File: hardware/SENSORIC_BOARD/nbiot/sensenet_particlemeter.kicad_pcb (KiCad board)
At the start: 2 copper layers, 63.6 x 72.3 mm, 80 parts, among them J1 CONN_01X01, J11 CONN_01X01, J13 BARREL_JACK, J17 CONN_01X01, J18 CONN_01X01, J19 CONN_01X01, J2 CONN_01X01, J20 CONN_01X01, J21 CONN_01X01, J3 CONN_01X01, J4 CONN_01X01, J5 CONN_01X01, J6 CONN_01X01, J9 CONN_01X01, P1 SMA_mini, P2 SMA_mini, P3 CONN_02X11, P4 USB_B, Q1 Q_NMOS_GSD, SW1 SW_Push, SW2 SW_DIP_x02, U1 MC33063, U10 bme280_barebone, U2 stm32f072, U3 QUECTEL_BC95, U4 SIM, U5 CAT24C02, U7 M10578-A2, U8 LD39050, Y1 8MHz

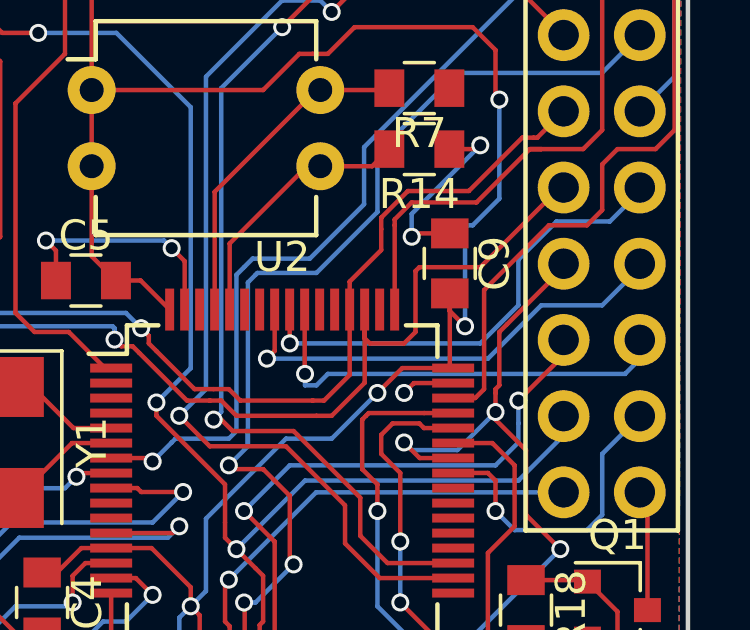
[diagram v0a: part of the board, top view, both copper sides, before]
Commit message: Zaklad nove verze je hotovy, ted jdu udelat vetsi zmeny v napajeni a layoutu, priprava na shield atd.
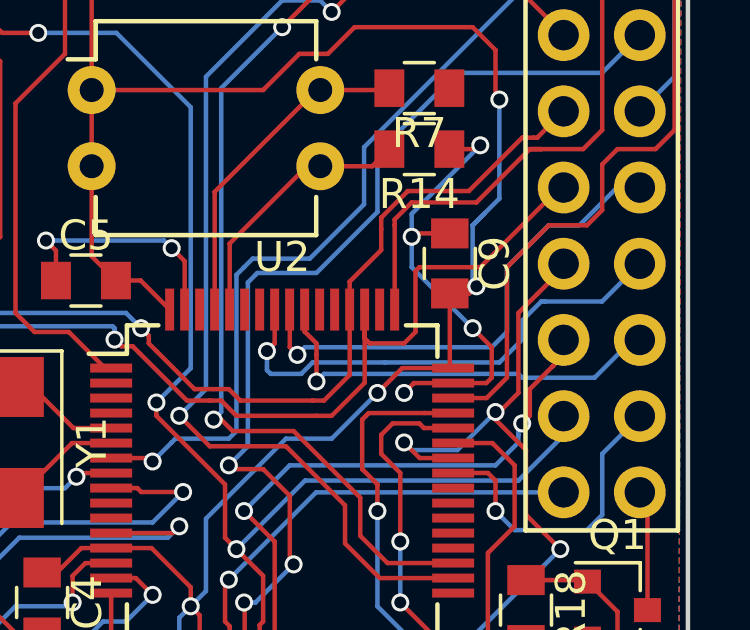
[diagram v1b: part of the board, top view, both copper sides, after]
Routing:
- net GND: track 262.0 -> 269.2 mm, vias 29 -> 30
- net +3V3: track 212.4 -> 211.1 mm
- net PM_SDI: track 15.6 -> 16.6 mm
- net PM_SDO: track 15.9 -> 16.7 mm
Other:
- net class Default: trace_width 0.5 -> 0.15
